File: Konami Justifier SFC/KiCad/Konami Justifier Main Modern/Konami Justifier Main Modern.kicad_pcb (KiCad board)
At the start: 4 copper layers, 25.2 x 50 mm, 19 parts, among them J1 RJ12, J2 Conn_01x06_Socket, U1 74VHC9164FT

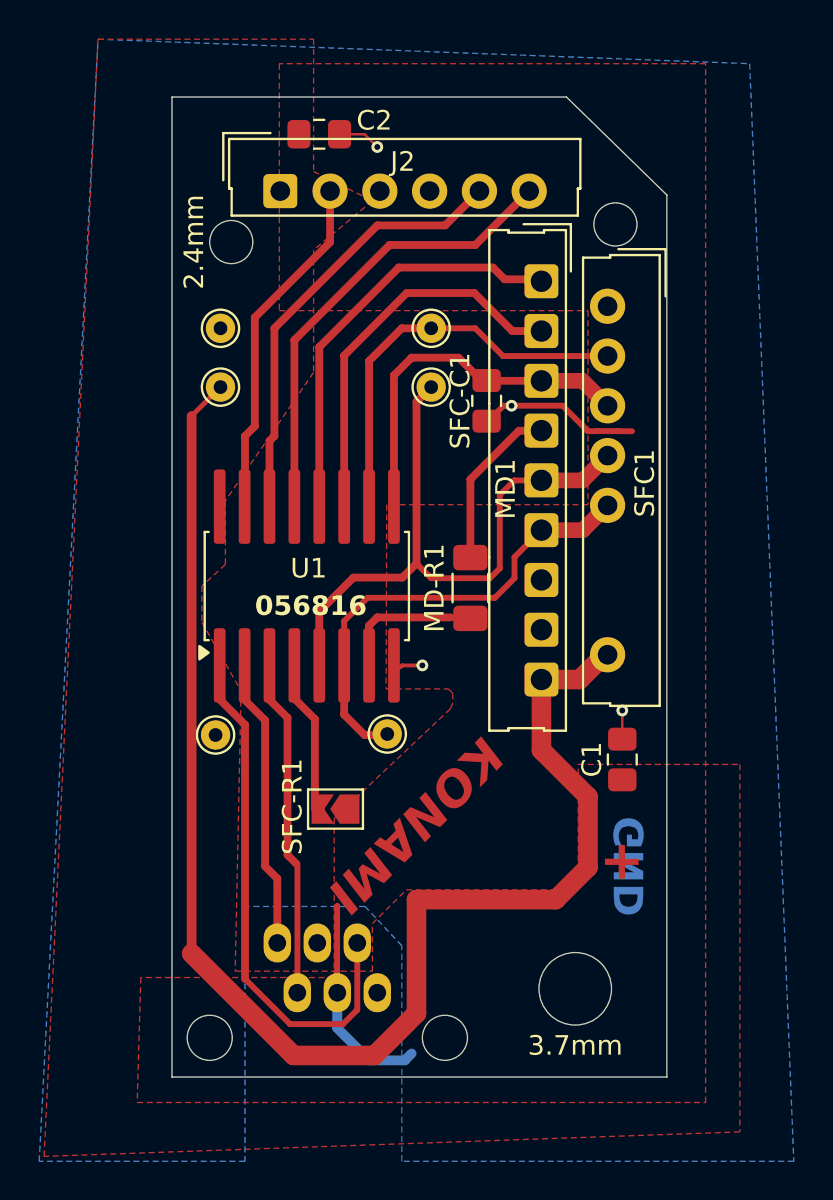
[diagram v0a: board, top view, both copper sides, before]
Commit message: Add files via upload
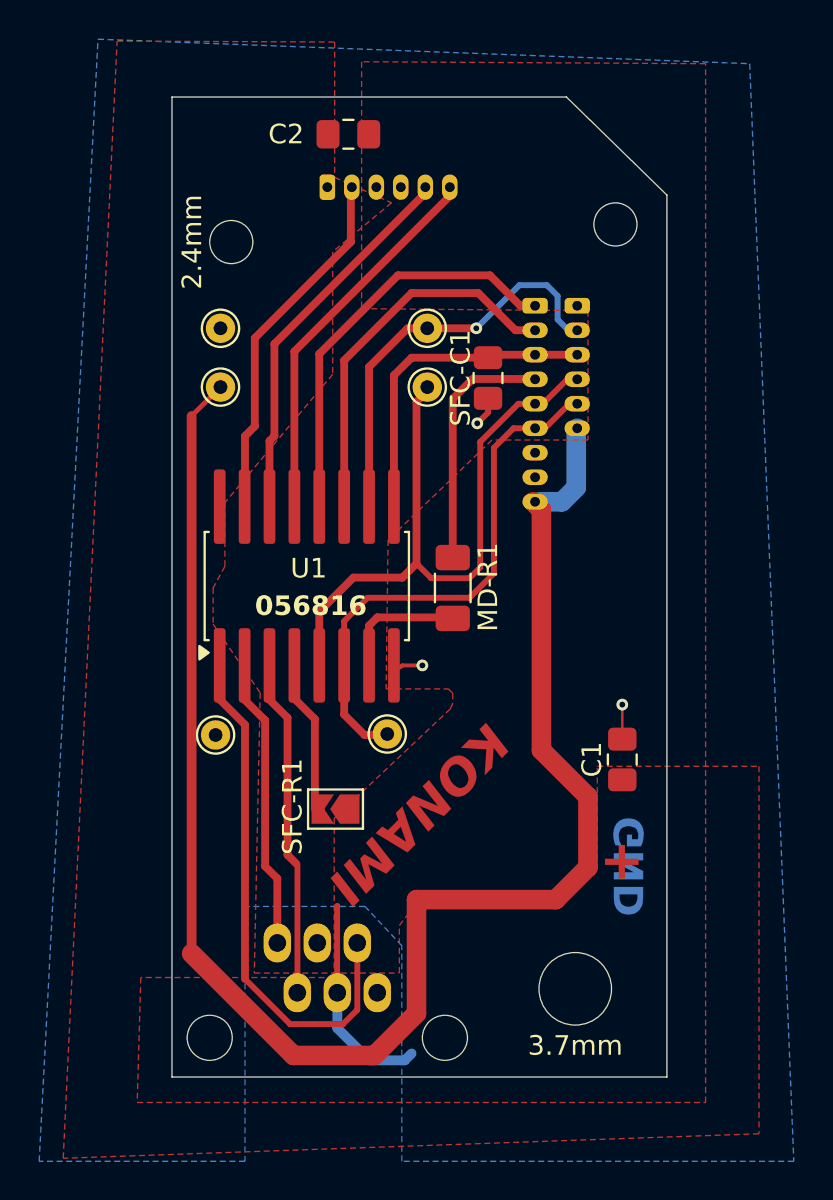
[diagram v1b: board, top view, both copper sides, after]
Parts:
- J2: footprint Connector_Molex:Molex_SL_171971-0006_1x06_P2.54mm_Vertical -> Connector_Molex:Molex_PicoBlade_53048-0610_1x06_P1.25mm_Horizontal; moved to B.Cu
- MD1: footprint Connector_Molex:Molex_SL_171971-0009_1x09_P2.54mm_Vertical -> Connector_Molex:Molex_PicoBlade_53047-0910_1x09_P1.25mm_Vertical; moved to B.Cu
- SFC1: value Conn_01x08_Pin -> Conn_01x06_Socket; footprint Connector_Molex:Molex_SL_171971-0008_1x08_P2.54mm_Vertical -> Connector_Molex:Molex_PicoBlade_53048-0610_1x06_P1.25mm_Horizontal; moved to B.Cu
- moved J2 2.41 mm to (147.7, 81.3)
- moved SFC1 1.55 mm to (160.4, 87.3)
- moved C2 1.49 mm to (148.8, 78.6)
- moved MD1 1.29 mm to (158.3, 87.3)
- moved SFC-C1 1.17 mm to (155.9, 91.0)
- moved MD-R1 0.90 mm to (154.1, 101.8)
- moved SFC-TP1 0.20 mm to (152.8, 88.5)
- moved SFC-TP2 0.20 mm to (152.8, 91.5)
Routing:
- net +5V: track 73.8 -> 84.3 mm
- net GND: track 24.1 -> 15.4 mm, vias 4 -> 3
- net Net-(MD1-Pin_4): track 8.70 -> 13.6 mm
- net Net-(J2-Pin_6): track 24.4 -> 20.5 mm
- net Net-(MD1-Pin_3): track 20.2 -> 17.1 mm
- net Net-(MD1-Pin_6): track 24.6 -> 27.6 mm
- net Net-(J2-Pin_5): track 23.4 -> 20.7 mm
- net Net-(J2-Pin_2): track 18.7 -> 19.4 mm
- net Net-(SFC1-Pin_2): track 21.7 -> 21.9 mm, vias 0 -> 1
